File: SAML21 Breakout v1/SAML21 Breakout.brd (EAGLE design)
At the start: 100 x 80 mm, 41 parts, among them J1 M50-4910545, U1 AT-SAM-L21-JTQFP, U2 AP7361C-33E-13, U3 MCP1501-CHY, Y2 32.768MHz

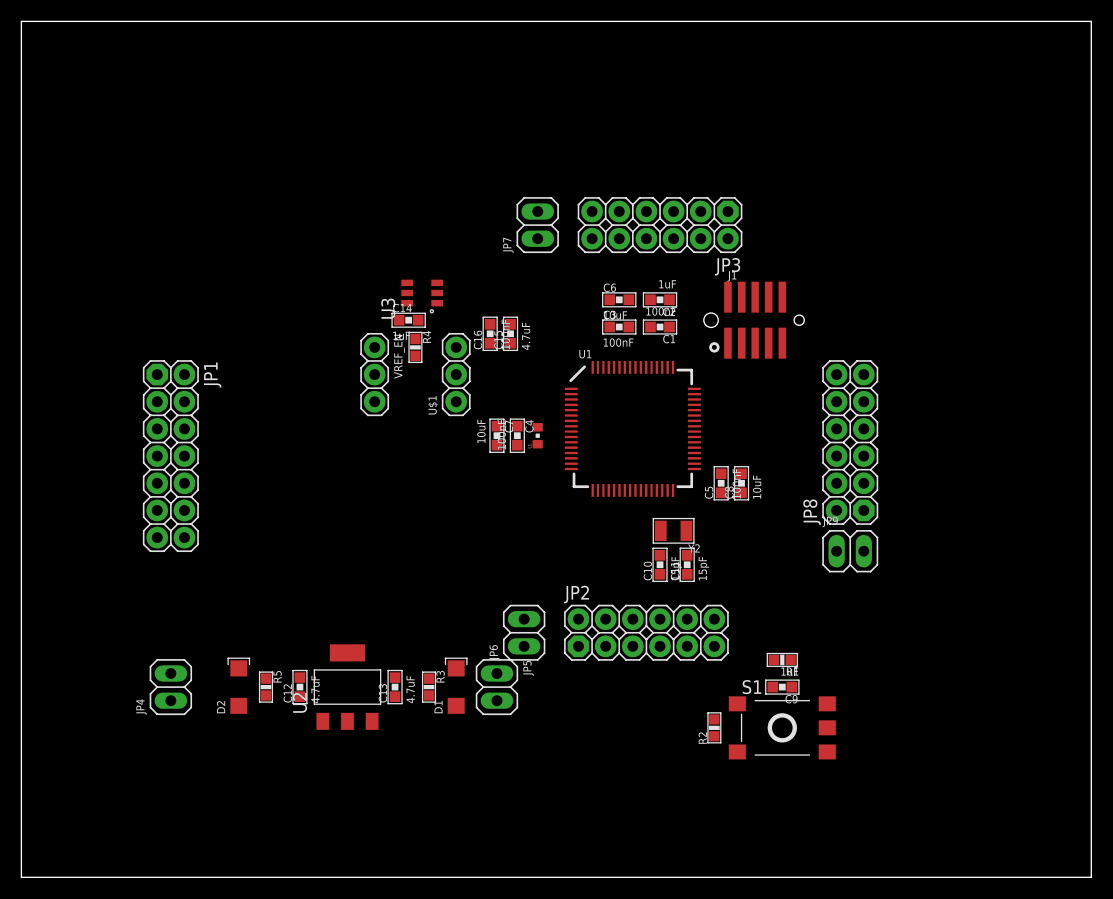
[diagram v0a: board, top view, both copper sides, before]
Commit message: ddx
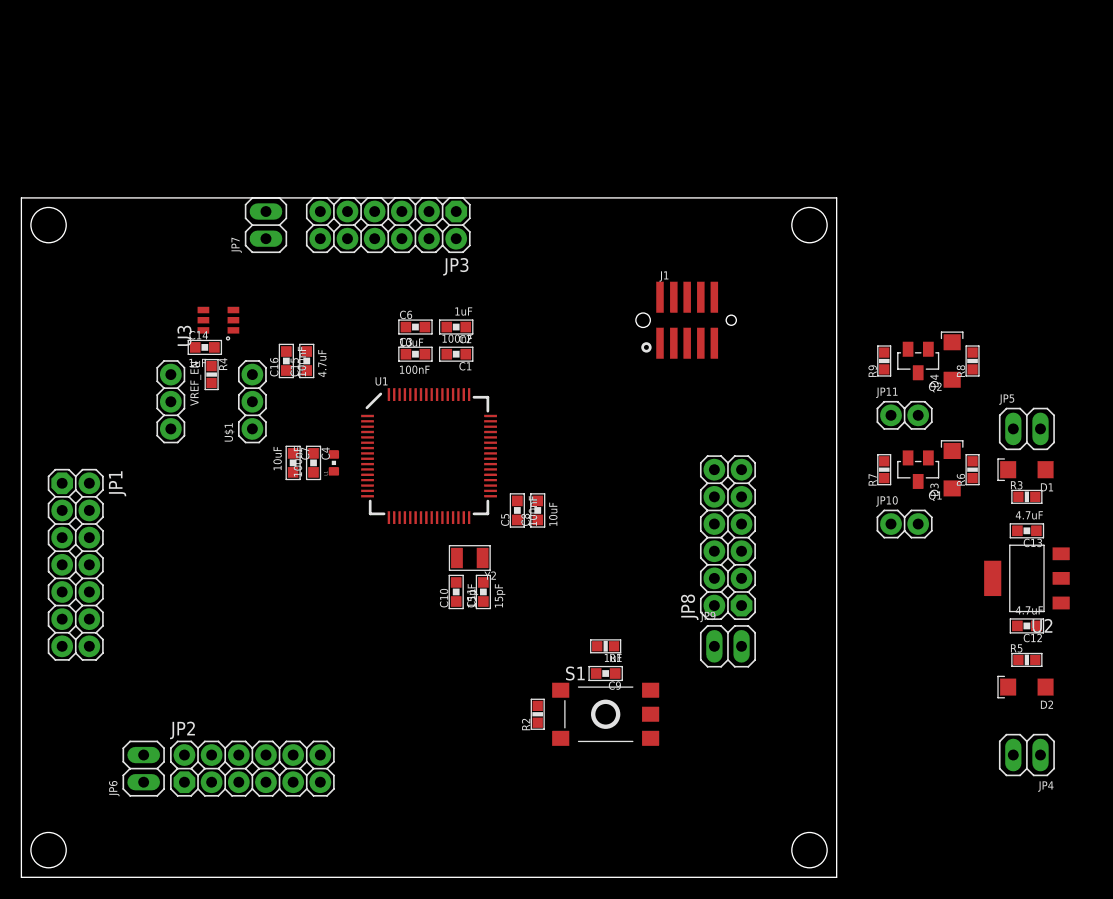
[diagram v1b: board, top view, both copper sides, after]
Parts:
- added D3, D4: PWR, dr-library:LED-1206
- added JP10, JP11: M02, dr-library:1X02
- added Q1, Q2: 2N7002, dr-library:SOT-23-3
- added R6, R8: 330, dr-library:RES-0603
- added R7, R9: 10k, dr-library:RES-0603
- added U$2, U$3, U$4, U$5: (no value), EmbeddedAdventures 3:STAND-OFF-HOLE
- moved JP4 80.3 mm to (94.0, 11.4), turned to 180 degrees
- moved D2 73.7 mm to (94.0, 17.8), turned to 180 degrees
- moved R5 71.2 mm to (94.0, 20.3), turned to 0 degrees
- moved C12 68.2 mm to (94.0, 23.5), turned to 180 degrees
- moved U2 64.3 mm to (94.0, 27.9), turned to 90 degrees
- moved C13 60.8 mm to (94.0, 32.4), turned to 180 degrees
- moved R3 58.6 mm to (94.0, 35.6), turned to 0 degrees
- moved D1 57.1 mm to (94.0, 38.1), turned to 180 degrees
- moved JP5 55.1 mm to (94.0, 41.9), turned to 0 degrees
- moved JP2 39.0 mm to (16.5, 11.4)
- moved JP6 37.8 mm to (11.4, 10.2)
- moved JP3 25.4 mm to (39.4, 59.7)
- moved JP7 25.4 mm to (22.9, 61.0)
- moved C3 19.2 mm to (36.8, 48.9)
- moved C5 19.2 mm to (46.4, 34.3)
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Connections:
- new net HEART: JP10.2, Q1.D, R7.1
- new net HEART2: JP11.2, Q2.D, R9.1
- new net N$10: D4.A, R8.1
- new net N$11: D4.C, Q2.G
- new net N$8: D3.A, R6.1
- new net N$9: D3.C, Q1.G
- net +3V3: now also R6.2, R8.2
- net GND: now also Q1.S, Q2.S, R7.2, R9.2
- net PA8: now also JP10.1
- net PB10: now also JP11.1
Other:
- board size 100 x 80 mm -> 76.2 x 63.5 mm
